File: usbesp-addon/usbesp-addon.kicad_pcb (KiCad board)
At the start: 2 copper layers, 20.3 x 10.2 mm, 7 parts, among them J2 Conn_01x04, J3 Conn_01x04, Q1 BC847BS, U1 FT232RL

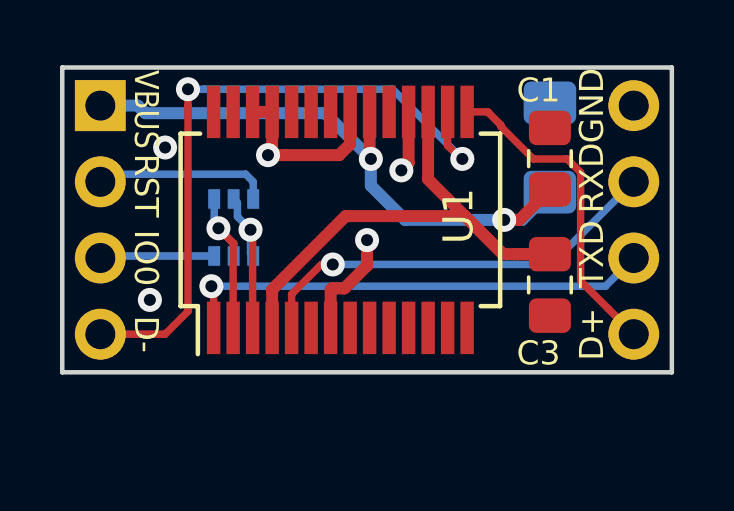
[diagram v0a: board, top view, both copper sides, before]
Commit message: PCB update
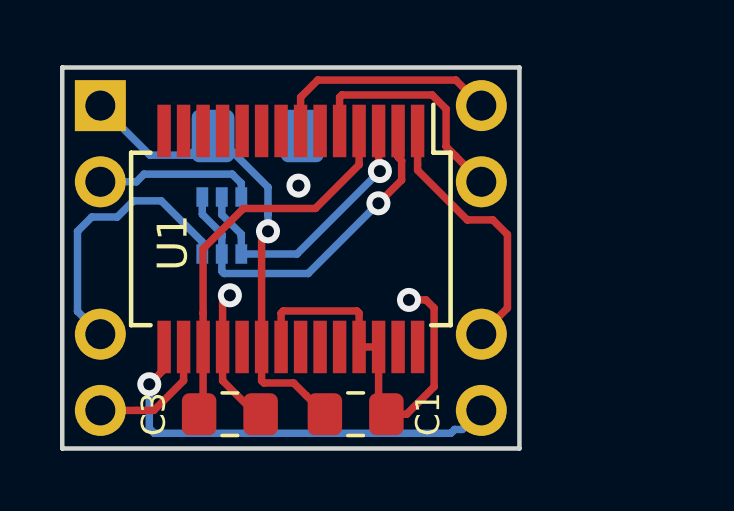
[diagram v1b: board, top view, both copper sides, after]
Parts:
- added J1: Conn_01x02, Connector_PinHeader_2.54mm:PinHeader_1x02_P2.54mm_Vertical, B.Cu at (142.2, 106.7)
- added J4: Conn_01x02, Connector_PinHeader_2.54mm:PinHeader_1x02_P2.54mm_Vertical, B.Cu at (154.9, 106.7)
- J2, J3: value Conn_01x04 -> Conn_01x02; footprint Connector_PinHeader_2.54mm:PinHeader_1x04_P2.54mm_Vertical -> Connector_PinHeader_2.54mm:PinHeader_1x02_P2.54mm_Vertical
- moved C3 11.5 mm to (146.6, 109.3), turned to 0 degrees
- moved C1 10.7 mm to (150.7, 109.3), turned to 0 degrees
- moved C2 9.75 mm to (147.5, 100.1), turned to 0 degrees
- moved J3 5.08 mm to (154.9, 99.1)
- moved U1 1.77 mm to (148.6, 103.5), turned to 270 degrees
- moved Q1 0.40 mm to (146.3, 103.1)
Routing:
- net /USBDM: track 22.5 -> 4.31 mm, vias 2 -> 0
- net GND: track 11.8 -> 25.9 mm, vias 5 -> 3
- net /TXD: track 15.9 -> 8.87 mm, vias 1 -> 0
- net /RXD: track 14.1 -> 7.82 mm, vias 1 -> 0
- net /DTR: track 5.69 -> 11.7 mm
- net /3v3: track 18.9 -> 13.1 mm
- net /IO0: track 3.82 -> 9.30 mm
- net /VBUS: track 21.0 -> 16.5 mm, vias 2 -> 1
- net /RTS: track 5.47 -> 9.29 mm
- net /USBDP: track 10.8 -> 14.4 mm, vias 0 -> 1
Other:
- board size 20.3 x 10.2 mm -> 15.2 x 12.7 mm
- net class Power removed
- board text removed: "USB-SERIAL ADDON"
